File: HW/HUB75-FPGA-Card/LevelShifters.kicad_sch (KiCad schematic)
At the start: 12 parts, among them J1 Conn_02x08_Odd_Even, J2 Conn_02x08_Odd_Even, J3 Conn_01x03, J4 Conn_01x03, J5 Conn_01x03, J6 Conn_01x03, U2 74AHCT245PW, U3 74AHCT245PW, U4 74AHCT245PW

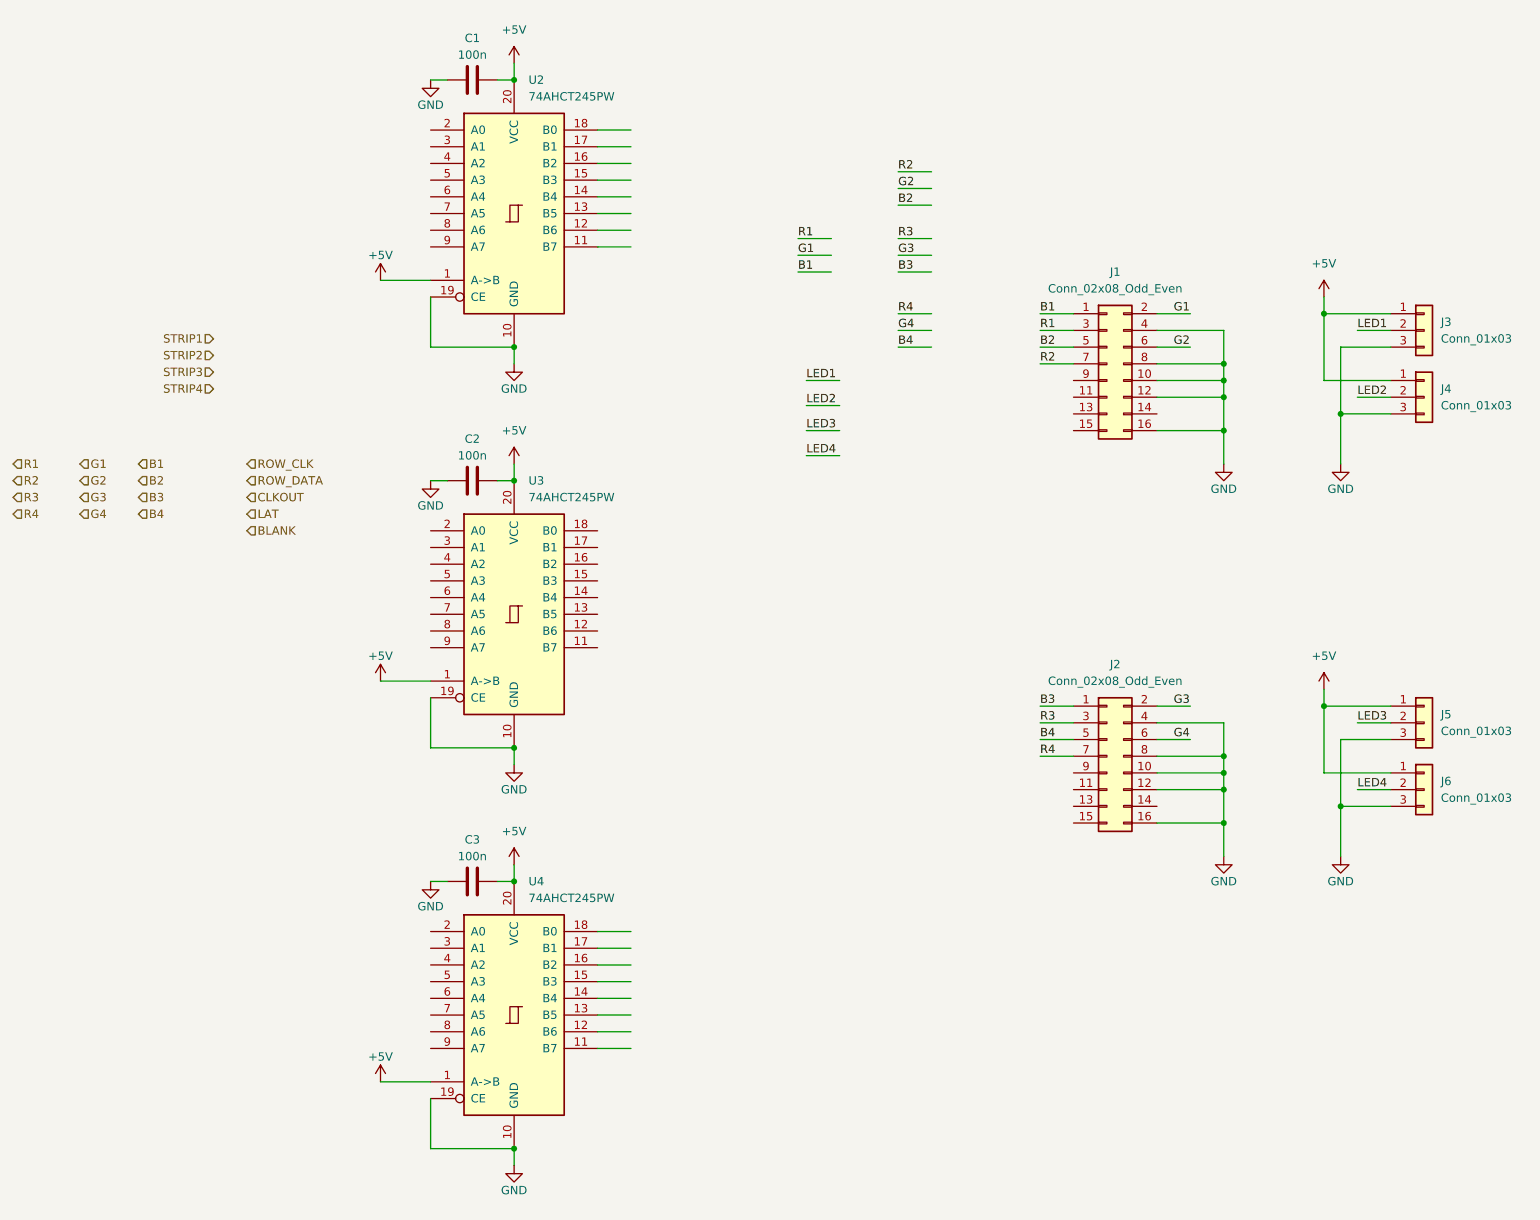
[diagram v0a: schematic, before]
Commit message: finish up schematic and begin routing
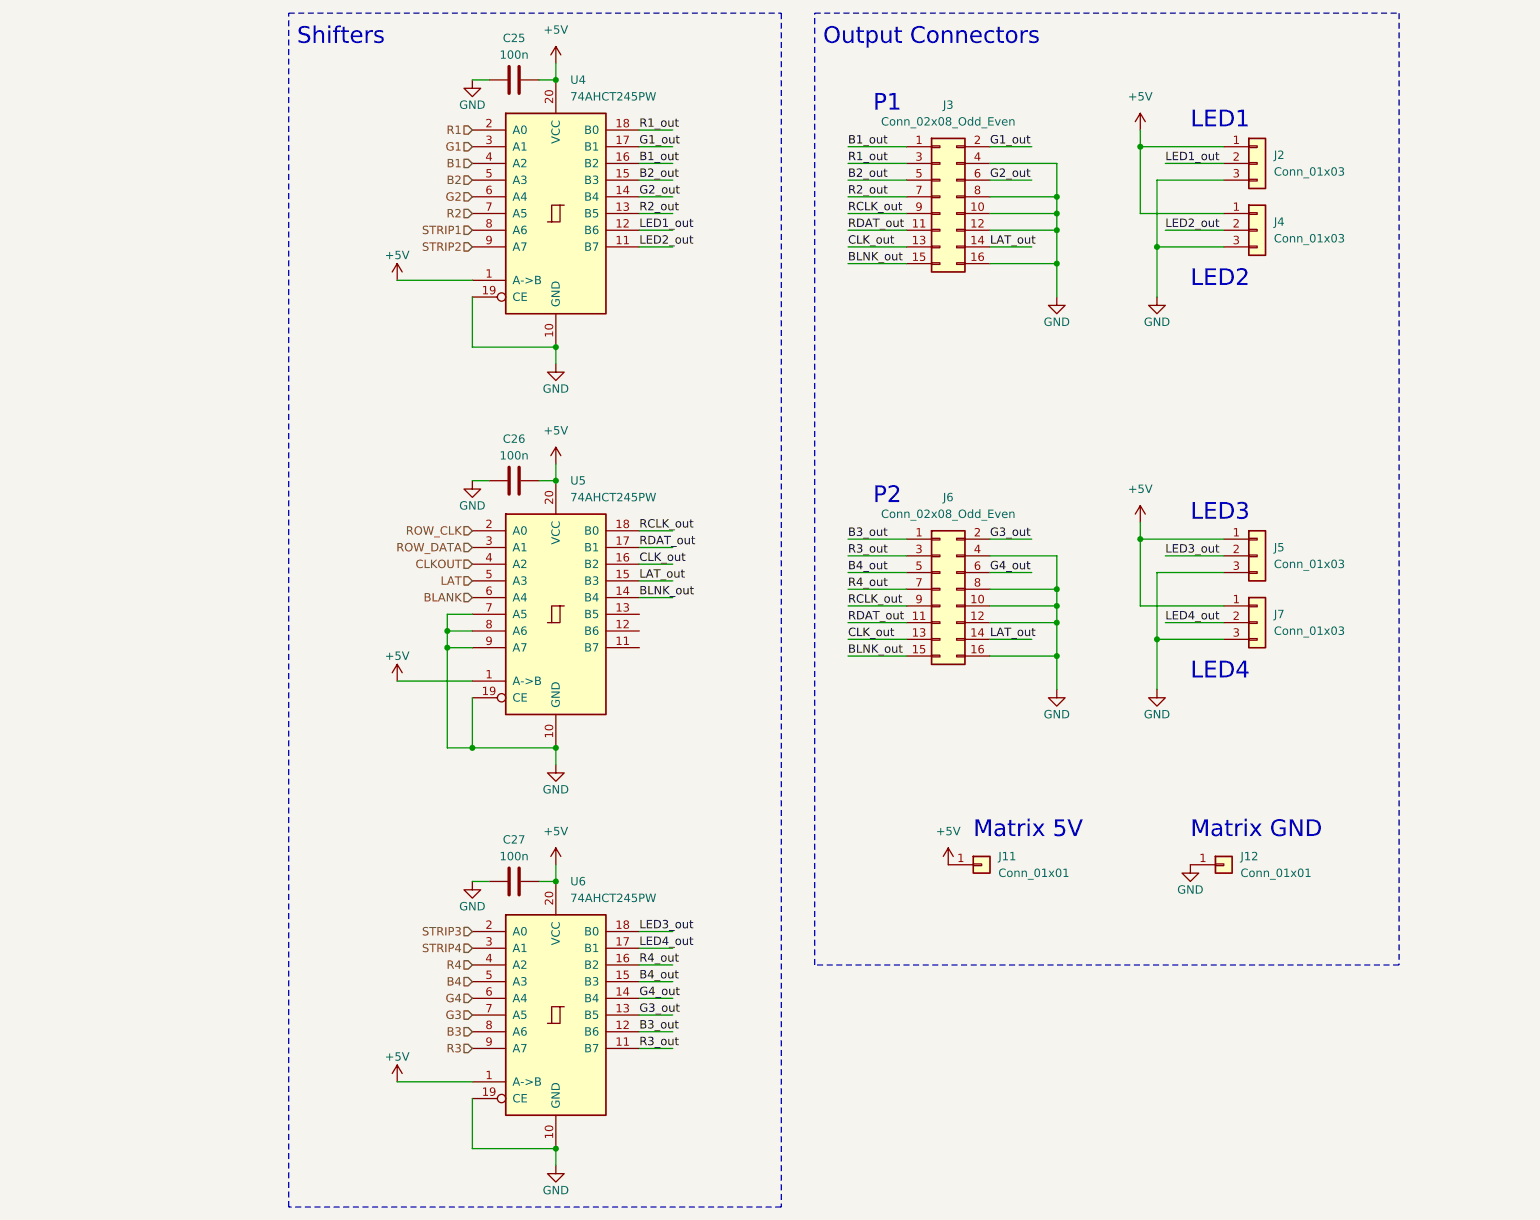
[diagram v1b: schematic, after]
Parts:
- added J11, J12: Conn_01x01, Connector_Wire:SolderWire-2sqmm_1x01_D2mm_OD3.9mm, symbol Connector_Generic:Conn_01x01
- C25: renamed from C1; footprint (none) -> Capacitor_SMD:C_0603_1608Metric
- C26: renamed from C2; footprint (none) -> Capacitor_SMD:C_0603_1608Metric
- C27: renamed from C3; footprint (none) -> Capacitor_SMD:C_0603_1608Metric
- J2: renamed from J3; footprint (none) -> Connector_PinHeader_2.54mm:PinHeader_1x03_P2.54mm_Vertical
- J4, J5: footprint (none) -> Connector_PinHeader_2.54mm:PinHeader_1x03_P2.54mm_Vertical
- J7: renamed from J6; footprint (none) -> Connector_PinHeader_2.54mm:PinHeader_1x03_P2.54mm_Vertical
- renumbered J1 to J3, J2 to J6, U2 to U4, U3 to U5, U4 to U6
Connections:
- net LED1 is gone; now on net LED1_out: J2.2 (Pin_2)
- net LED2 is gone; now on net LED2_out: J4.2 (Pin_2)
- net LED3 is gone; now on net LED3_out: J5.2 (Pin_2)
- net LED4 is gone; now on net LED4_out: J7.2 (Pin_2)
- net +5V: now also J11.1 (Pin_1)
- net B1: now also U4.4 (A2); no longer J3.1 (Pin_1)
- net B2: now also U4.5 (A3); no longer J3.5 (Pin_5)
- net B3: now also U6.8 (A6); no longer J6.1 (Pin_1)
- net B4: now also U6.5 (A3); no longer J6.5 (Pin_5)
- net BLANK: now also U5.6 (A4)
- net CLKOUT: now also U5.4 (A2)
- net G1: now also U4.3 (A1); no longer J3.2 (Pin_2)
- net G2: now also U4.6 (A4); no longer J3.6 (Pin_6)
- net G3: now also U6.7 (A5); no longer J6.2 (Pin_2)
- net G4: now also U6.6 (A4); no longer J6.6 (Pin_6)
- net GND: now also U5.7 (A5), U5.8 (A6), U5.9 (A7), J12.1 (Pin_1)
- net LAT: now also U5.5 (A3)
- net R1: now also U4.2 (A0); no longer J3.3 (Pin_3)
- net R2: now also U4.7 (A5); no longer J3.7 (Pin_7)
- net R3: now also U6.9 (A7); no longer J6.3 (Pin_3)
- net R4: now also U6.4 (A2); no longer J6.7 (Pin_7)
- net ROW_CLK: now also U5.2 (A0)
- net ROW_DATA: now also U5.3 (A1)
- net STRIP1: now also U4.8 (A6)
- net STRIP2: now also U4.9 (A7)
- net STRIP3: now also U6.2 (A0)
- net STRIP4: now also U6.3 (A1)
- net RDAT_out: now reaches J3.11 (Pin_11)
- net RDAT_out: now also J6.11 (Pin_11), U5.17 (B1)
- net CLK_out: now reaches J3.13 (Pin_13)
- net CLK_out: now also J6.13 (Pin_13), U5.16 (B2)
- net LAT_out: now reaches J3.14 (Pin_14)
- net LAT_out: now also J6.14 (Pin_14), U5.15 (B3)
- net BLNK_out: now reaches J3.15 (Pin_15)
- net BLNK_out: now also J6.15 (Pin_15), U5.14 (B4)
- net RCLK_out: now reaches J3.9 (Pin_9)
- net RCLK_out: now also J6.9 (Pin_9), U5.18 (B0)
- net R3_out: now reaches U6.11 (B7)
- net R3_out: now also J6.3 (Pin_3)
- net B3_out: now reaches U6.12 (B6)
- net B3_out: now also J6.1 (Pin_1)
- net G3_out: now reaches U6.13 (B5)
- net G3_out: now also J6.2 (Pin_2)
- net G4_out: now reaches U6.14 (B4)
- net G4_out: now also J6.6 (Pin_6)
- net B4_out: now reaches U6.15 (B3)
- net B4_out: now also J6.5 (Pin_5)
- net R4_out: now reaches U6.16 (B2)
- net R4_out: now also J6.7 (Pin_7)
- net LED4_out: now reaches U6.17 (B1)
- net LED3_out: now reaches U6.18 (B0)
- net LED2_out: now reaches U4.11 (B7)
- net LED1_out: now reaches U4.12 (B6)
- net R2_out: now reaches U4.13 (B5)
- net R2_out: now also J3.7 (Pin_7)
- net G2_out: now reaches U4.14 (B4)
- net G2_out: now also J3.6 (Pin_6)
- net B2_out: now reaches U4.15 (B3)
- net B2_out: now also J3.5 (Pin_5)
- net B1_out: now reaches U4.16 (B2)
- net B1_out: now also J3.1 (Pin_1)
- net G1_out: now reaches U4.17 (B1)
- net G1_out: now also J3.2 (Pin_2)
- net R1_out: now reaches U4.18 (B0)
- net R1_out: now also J3.3 (Pin_3)
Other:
- note added: "LED1"
- note added: "LED2"
- note added: "LED3"
- note added: "LED4"
- note added: "Matrix 5V"
- note added: "Matrix GND"
- note added: "Output Connectors"
- note added: "P1"
- note added: "P2"
- note added: "Shifters"
- moved on the sheet: C25, C26, C27, J2, J3, J4, J5, J6, J7, U4, U5, U6
